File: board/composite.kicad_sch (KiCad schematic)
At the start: 18 parts, among them J6 COMPOSITE, U17 CPST, U18 74HC373, U19 74HC373, U20 74HC165, U21 74HC165, Y1 14.318MHz

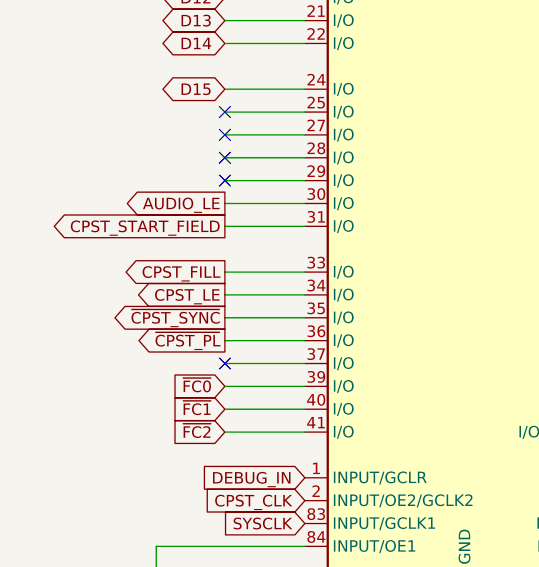
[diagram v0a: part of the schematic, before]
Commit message: checkpoint
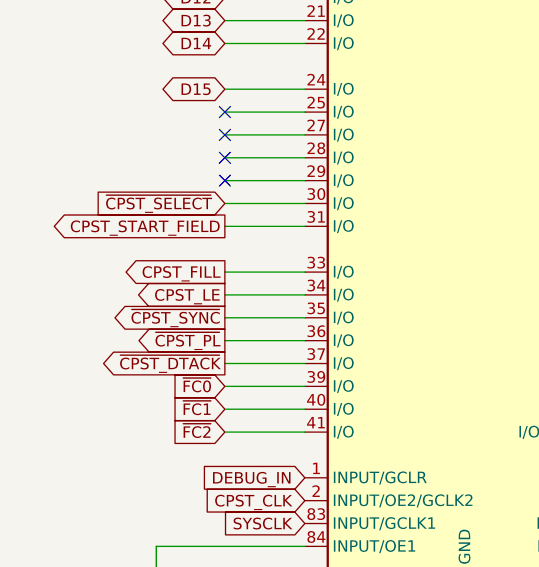
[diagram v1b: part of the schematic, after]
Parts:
- U20, U21: footprint Package_DIP:DIP-20_W7.62mm -> Package_DIP:DIP-16_W7.62mm
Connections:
- net ~{CPST_DTACK}: now reaches U17.37 (I/O)
- net AUDIO_LE renamed ~{CPST_SELECT}
- no-connect marks 7 -> 6
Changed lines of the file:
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@@
 	)
 	(no_connect
-		(at 34.29 138.43)
-	)
-	(no_connect
 		(at 34.29 118.11)
 	)
@@
 		)
 	)
-	(global_label "AUDIO_LE"
-		(shape output)
-		(at 34.29 120.65 180)
-		(fields_autoplaced yes)
-		(effects
-			(font
-				(size 1.27 1.27)
-			)
-			(justify right)
-		)
-		(property "Intersheetrefs" "${INTERSHEET_REFS}"
-			(at 22.5357 120.65 0)
-			(effects
-				(font
-					(size 1.27 1.27)
-				)
-				(justify right)
-				(hide yes)
-			)
-		)
-	)
 	(global_label "CPST_TDI"
 		(shape input)
@@
 		)
 	)
+	(global_label "~{CPST_SELECT}"
+		(shape input)
+		(at 34.29 120.65 180)
+		(fields_autoplaced yes)
+		(effects
+			(font
+				(size 1.27 1.27)
+			)
+			(justify right)
+		)
+		(property "Intersheetrefs" "${INTERSHEET_REFS}"
+			(at 18.8469 120.65 0)
+			(effects
+				(font
+					(size 1.27 1.27)
+				)
+				(justify right)
+				(hide yes)
+			)
+		)
+	)
 	(global_label "D6"
 		(shape input)
@@
 		)
 	)
+	(global_label "~{CPST_DTACK}"
+		(shape output)
+		(at 34.29 138.43 180)
+		(fields_autoplaced yes)
+		(effects
+			(font
+				(size 1.27 1.27)
+			)
+			(justify right)
+		)
+		(property "Intersheetrefs" "${INTERSHEET_REFS}"
+			(at 19.7539 138.43 0)
+			(effects
+				(font
+					(size 1.27 1.27)
+				)
+				(justify right)
+				(hide yes)
+			)
+		)
+	)
 	(global_label "A16"
 		(shape bidirectional)
@@
 			)
 		)
-		(property "Footprint" "Package_DIP:DIP-20_W7.62mm"
+		(property "Footprint" "Package_DIP:DIP-16_W7.62mm"
 			(at 181.61 119.38 0)
 			(effects
@@
 			)
 		)
-		(property "Footprint" "Package_DIP:DIP-20_W7.62mm"
+		(property "Footprint" "Package_DIP:DIP-16_W7.62mm"
 			(at 181.61 55.88 0)
 			(effects
